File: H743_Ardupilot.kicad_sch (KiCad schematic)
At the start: 8 parts, among them U1 USBLC6-2P6

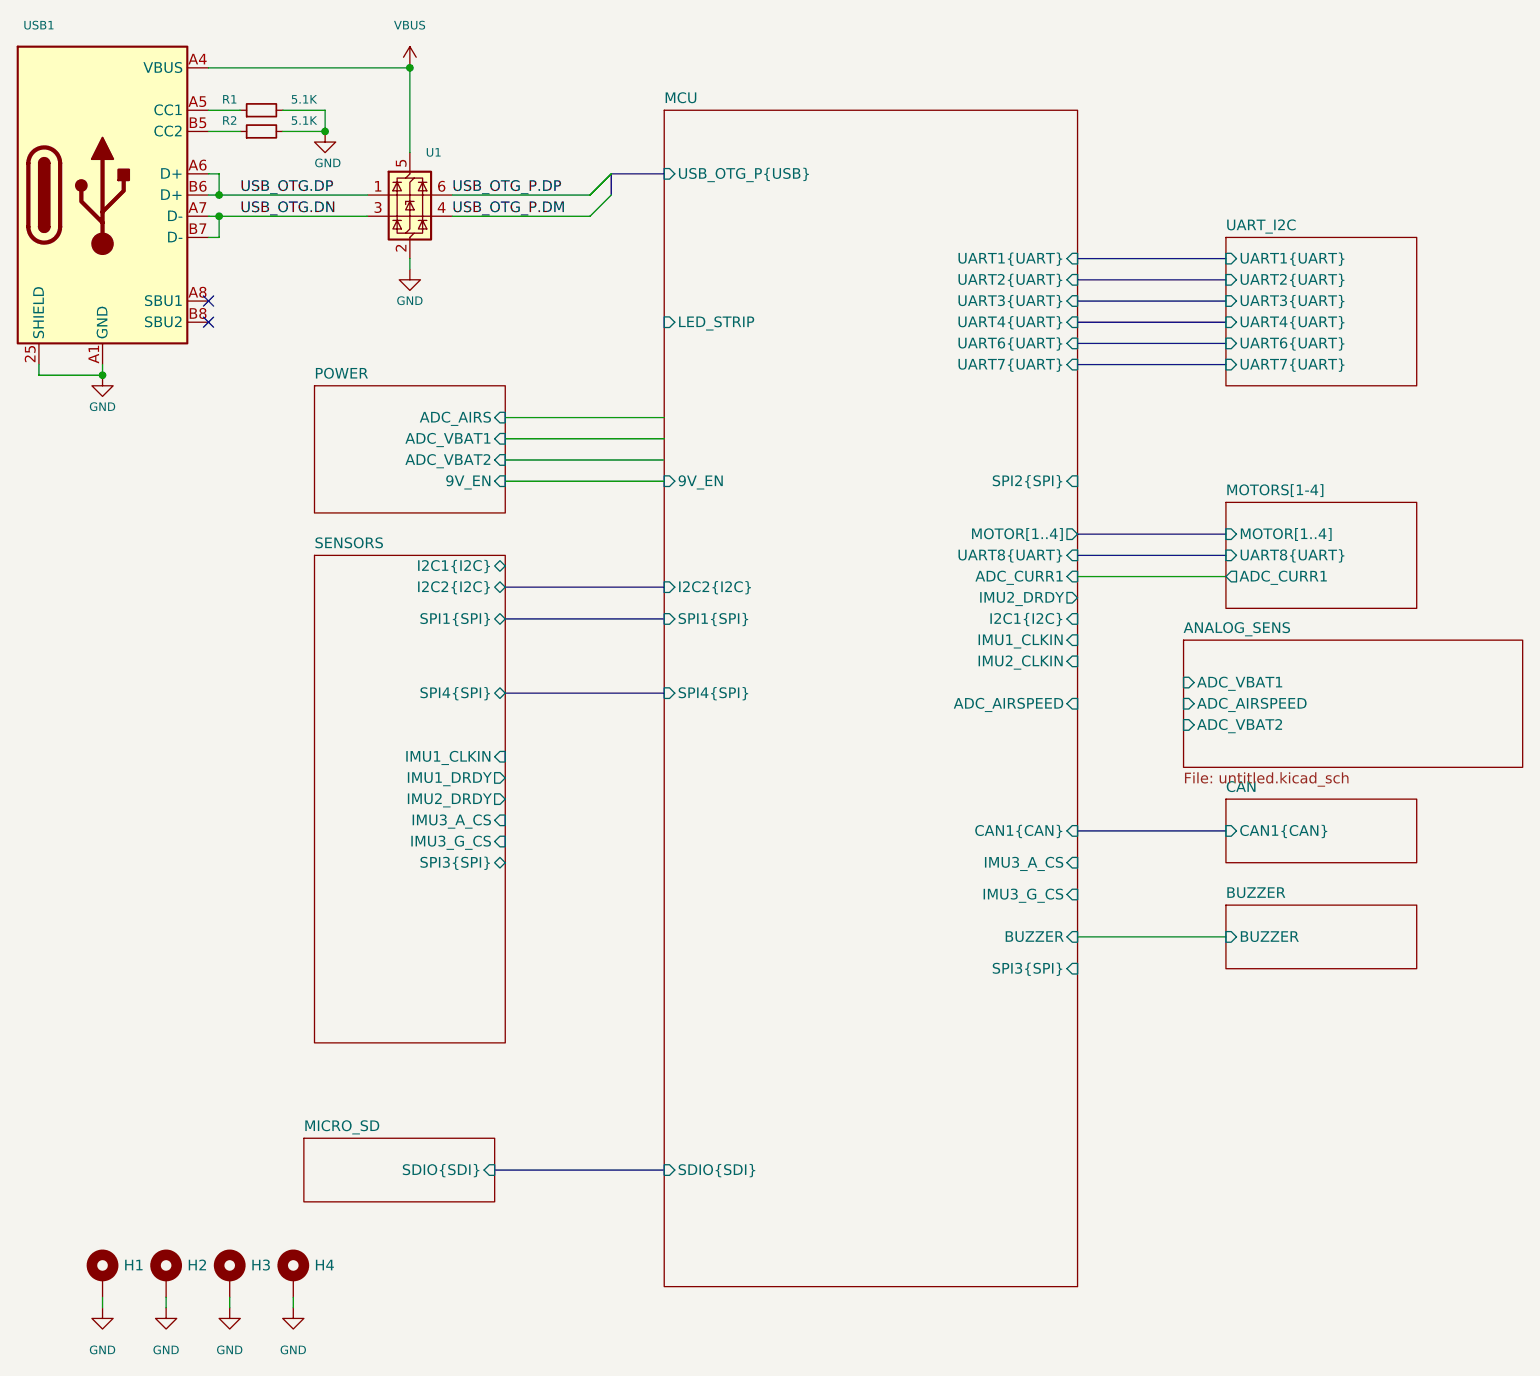
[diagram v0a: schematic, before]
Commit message: update 1
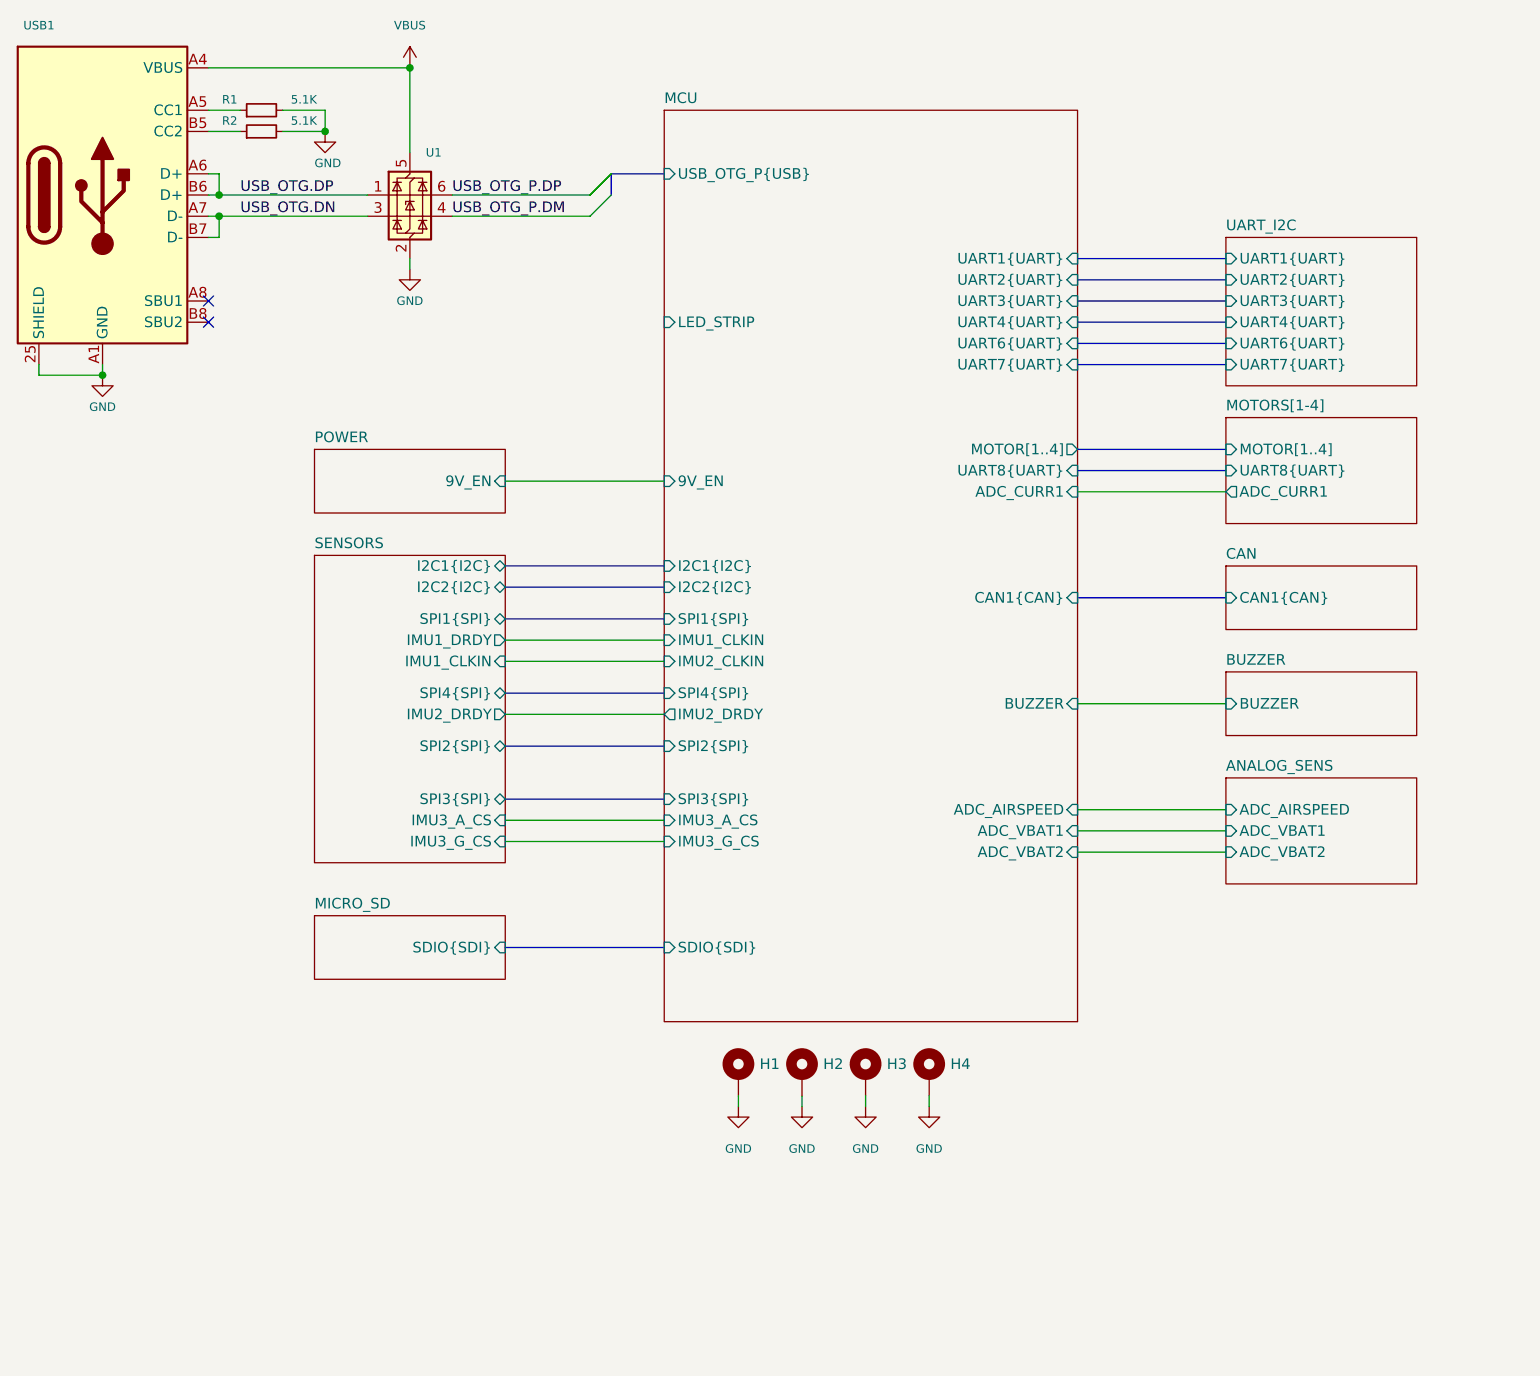
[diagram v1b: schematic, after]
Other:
- sheet MCU ports: added ADC_VBAT1, ADC_VBAT2; removed none
- sheet POWER ports: added none; removed ADC_AIRS, ADC_VBAT1, ADC_VBAT2
- sheet SENSORS ports: added SPI2{SPI}; removed none
- moved on the sheet: H1, H2, H3, H4
